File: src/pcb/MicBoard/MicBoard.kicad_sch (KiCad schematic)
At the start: 4 parts, among them J1 Conn_01x10_Pin

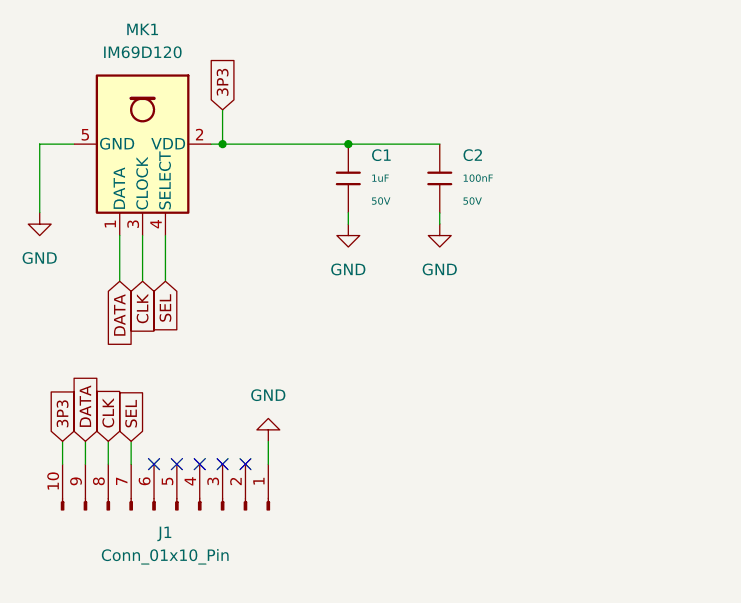
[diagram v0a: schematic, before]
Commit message: finalized lyout for microphone
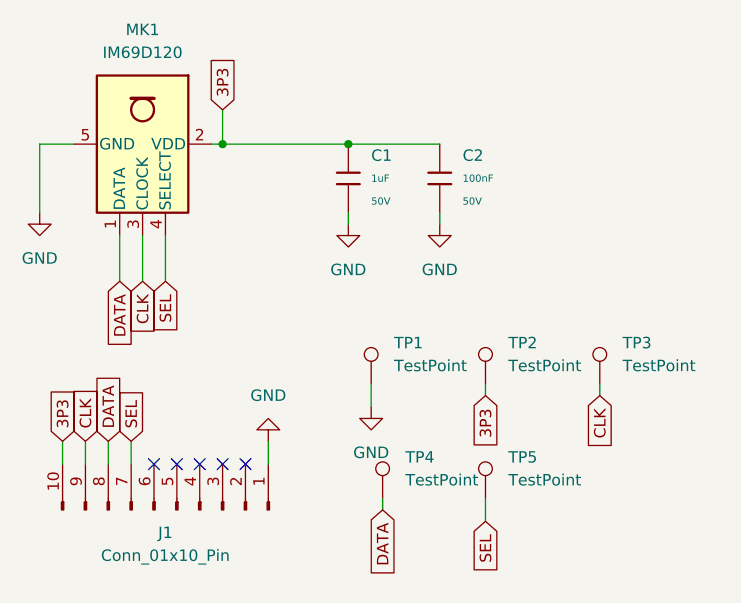
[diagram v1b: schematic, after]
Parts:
- added TP1, TP2, TP3, TP4, TP5: TestPoint, TestPoint:TestPoint_THTPad_D1.0mm_Drill0.5mm, symbol Connector:TestPoint
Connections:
- net 3P3: now also TP2.1
- net CLK: now also J1.9 (Pin_9), TP3.1; no longer J1.8 (Pin_8)
- net DATA: now also J1.8 (Pin_8), TP4.1; no longer J1.9 (Pin_9)
- net GND: now also TP1.1
- net SEL: now also TP5.1
